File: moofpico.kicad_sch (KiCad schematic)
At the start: 21 parts, among them J1 Serial, J2 Micro_SD_Card, J3 Bus_Apple_II_Card_Side, Q1 BS170, SW2 SW_DIP_x02, U1 Pico, U2 74LVC245, U3 74F11, U4 74LVC245, U5 74LVC245

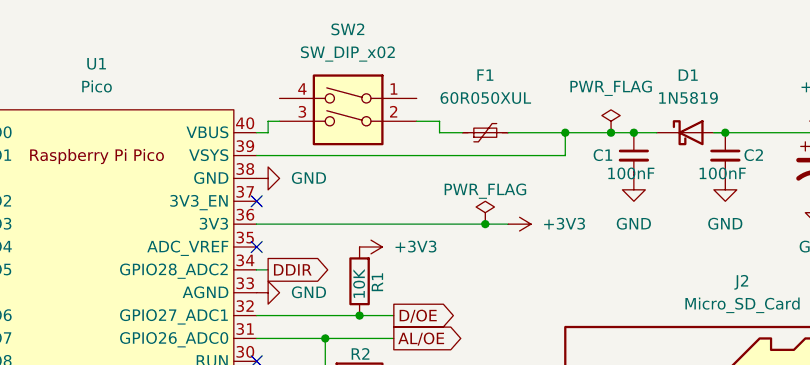
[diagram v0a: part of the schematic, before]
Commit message: resync w/ libraries
add fp/sym for MEM2061

pretty sure I can't redistribute the MEM2061 footprints, alas
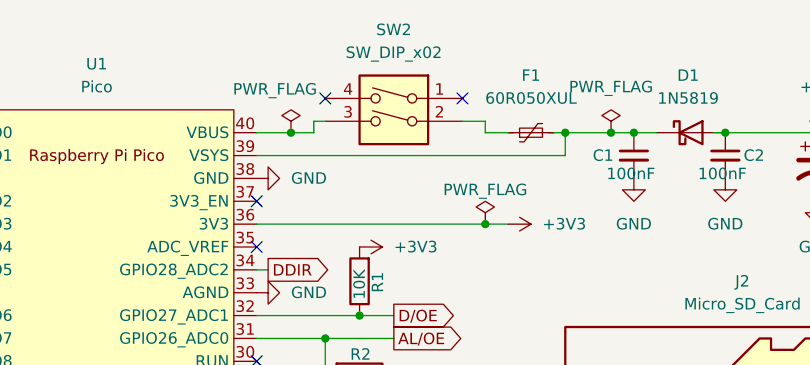
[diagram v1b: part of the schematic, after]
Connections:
- no-connect marks 32 -> 34
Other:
- moved on the sheet: F1, SW2
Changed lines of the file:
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@@
 	)
 	(junction
+		(at 170.18 29.21)
+		(diameter 0)
+		(color 0 0 0 0)
+	)
+	(junction
 		(at 110.49 171.45)
 		(diameter 0)
@@
 	)
 	(no_connect
+		(at 189.23 25.4)
+	)
+	(no_connect
 		(at 135.89 181.61)
 	)
@@
 	)
 	(no_connect
+		(at 173.99 25.4)
+	)
+	(no_connect
 		(at 161.29 179.07)
 	)
@@
 	(wire
 		(pts
-			(xy 184.15 27.94) (xy 186.69 27.94)
+			(xy 170.18 29.21) (xy 172.72 29.21)
+		)
+		(stroke
+			(width 0)
+			(type default)
+		)
+	)
+	(wire
+		(pts
+			(xy 189.23 27.94) (xy 191.77 27.94)
 		)
 		(stroke
@@
 	(wire
 		(pts
-			(xy 186.69 27.94) (xy 186.69 29.21)
+			(xy 191.77 27.94) (xy 191.77 29.21)
 		)
 		(stroke
@@
 	(wire
 		(pts
-			(xy 194.31 29.21) (xy 200.66 29.21)
-		)
-		(stroke
-			(width 0)
-			(type default)
-		)
-	)
-	(wire
-		(pts
 			(xy 166.37 57.15) (xy 173.99 57.15)
 		)
@@
 	(wire
 		(pts
-			(xy 167.64 27.94) (xy 168.91 27.94)
+			(xy 172.72 27.94) (xy 173.99 27.94)
 		)
 		(stroke
@@
 	(wire
 		(pts
-			(xy 167.64 27.94) (xy 167.64 29.21)
+			(xy 172.72 27.94) (xy 172.72 29.21)
 		)
 		(stroke
@@
 	(wire
 		(pts
-			(xy 167.64 29.21) (xy 166.37 29.21)
+			(xy 166.37 29.21) (xy 170.18 29.21)
 		)
 		(stroke
@@
 	(wire
 		(pts
+			(xy 199.39 29.21) (xy 200.66 29.21)
+		)
+		(stroke
+			(width 0)
+			(type default)
+		)
+	)
+	(wire
+		(pts
 			(xy 163.83 143.51) (xy 193.04 143.51)
 		)
@@
 	(wire
 		(pts
-			(xy 186.69 29.21) (xy 189.23 29.21)
+			(xy 191.77 29.21) (xy 194.31 29.21)
 		)
 		(stroke
@@
 	)
 	(symbol
+		(lib_id "power:PWR_FLAG")
+		(at 170.18 29.21 0)
+		(unit 1)
+		(exclude_from_sim no)
+		(in_bom yes)
+		(on_board yes)
+		(dnp no)
+		(property "Reference" "#FLG03"
+			(at 170.18 27.305 0)
+			(effects
+				(font
+					(size 1.27 1.27)
+				)
+				(hide yes)
+			)
+		)
+		(property "Value" "PWR_FLAG"
+			(at 168.402 24.384 0)
+			(effects
+				(font
+					(size 1.27 1.27)
+				)
+			)
+		)
+		(property "Footprint" ""
+			(at 170.18 29.21 0)
+			(effects
+				(font
+					(size 1.27 1.27)
+				)
+				(hide yes)
+			)
+		)
+		(property "Datasheet" "~"
+			(at 170.18 29.21 0)
+			(effects
+				(font
+					(size 1.27 1.27)
+				)
+				(hide yes)
+			)
+		)
+		(property "Description" "Special symbol for telling ERC where power comes from"
+			(at 170.18 29.21 0)
+			(effects
+				(font
+					(size 1.27 1.27)
+				)
+				(hide yes)
+			)
+		)
+		(pin "1"
+		)
+		(instances
+			(project "moofpico"
+				(path "/adf04048-7c47-4d7c-943c-c55ccf696419"
+					(reference "#FLG03")
+					(unit 1)
+				)
+			)
+		)
+	)
+	(symbol
 		(lib_id "power:GND")
 		(at 275.59 134.62 0)
@@
 	(symbol
 		(lib_id "Switch:SW_DIP_x02")
-		(at 176.53 27.94 0)
+		(at 181.61 27.94 0)
 		(mirror y)
 		(unit 1)
@@
 		(dnp no)
 		(property "Reference" "SW2"
-			(at 176.53 17.78 0)
+			(at 181.61 17.78 0)
 			(effects
 				(font
@@
 		)
 		(property "Value" "SW_DIP_x02"
-			(at 176.53 20.32 0)
+			(at 181.61 20.32 0)
 			(effects
 				(font
@@
 		)
 		(property "Footprint" "Button_Switch_THT:SW_DIP_SPSTx02_Slide_9.78x7.26mm_W7.62mm_P2.54mm"
-			(at 176.53 27.94 0)
+			(at 181.61 27.94 0)
 			(effects
 				(font
@@
 		)
 		(property "Datasheet" "https://www.mouser.com/datasheet/2/418/7/ENG_CD_1825360_B5-2021008.pdf"
-			(at 176.53 27.94 0)
+			(at 181.61 27.94 0)
 			(effects
 				(font
@@
 		)
 		(property "Description" "2x DIP Switch, Single Pole Single Throw (SPST) switch, small symbol"
-			(at 176.53 27.94 0)
+			(at 181.61 27.94 0)
 			(effects
 				(font
@@
 	(symbol
 		(lib_id "Device:Polyfuse_Small")
-		(at 191.77 29.21 90)
+		(at 196.85 29.21 90)
 		(unit 1)
 		(exclude_from_sim no)
@@
 		(on_board yes)
 		(dnp no)
-		(fields_autoplaced yes)
 		(property "Reference" "F1"
-			(at 191.77 22.86 90)
+			(at 196.85 22.86 90)
 			(effects
 				(font
@@
 		)
 		(property "Value" "60R050XUL"
-			(at 191.77 25.4 90)
+			(at 196.85 25.4 90)
 			(effects
 				(font
@@
 		)
 		(property "Footprint" "Fuse:Fuse_BelFuse_0ZRE0005FF_L8.3mm_W3.8mm"
-			(at 196.85 27.94 0)
+			(at 201.93 27.94 0)
 			(effects
 				(font
@@
 		)
 		(property "Datasheet" "~"
-			(at 191.77 29.21 0)
+			(at 196.85 29.21 0)
 			(effects
 				(font
@@
 		)
 		(property "Description" "Resettable fuse, polymeric positive temperature coefficient, small symbol"
-			(at 191.77 29.21 0)
+			(at 196.85 29.21 0)
 			(effects
 				(font
